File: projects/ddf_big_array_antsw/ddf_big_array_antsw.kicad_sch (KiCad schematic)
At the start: 35 parts, among them J1 Conn_Coaxial, J2 Conn_Coaxial, J3 Conn_Coaxial, J4 Conn_Coaxial, J5 Conn_Coaxial, J6 RJ45_Shielded

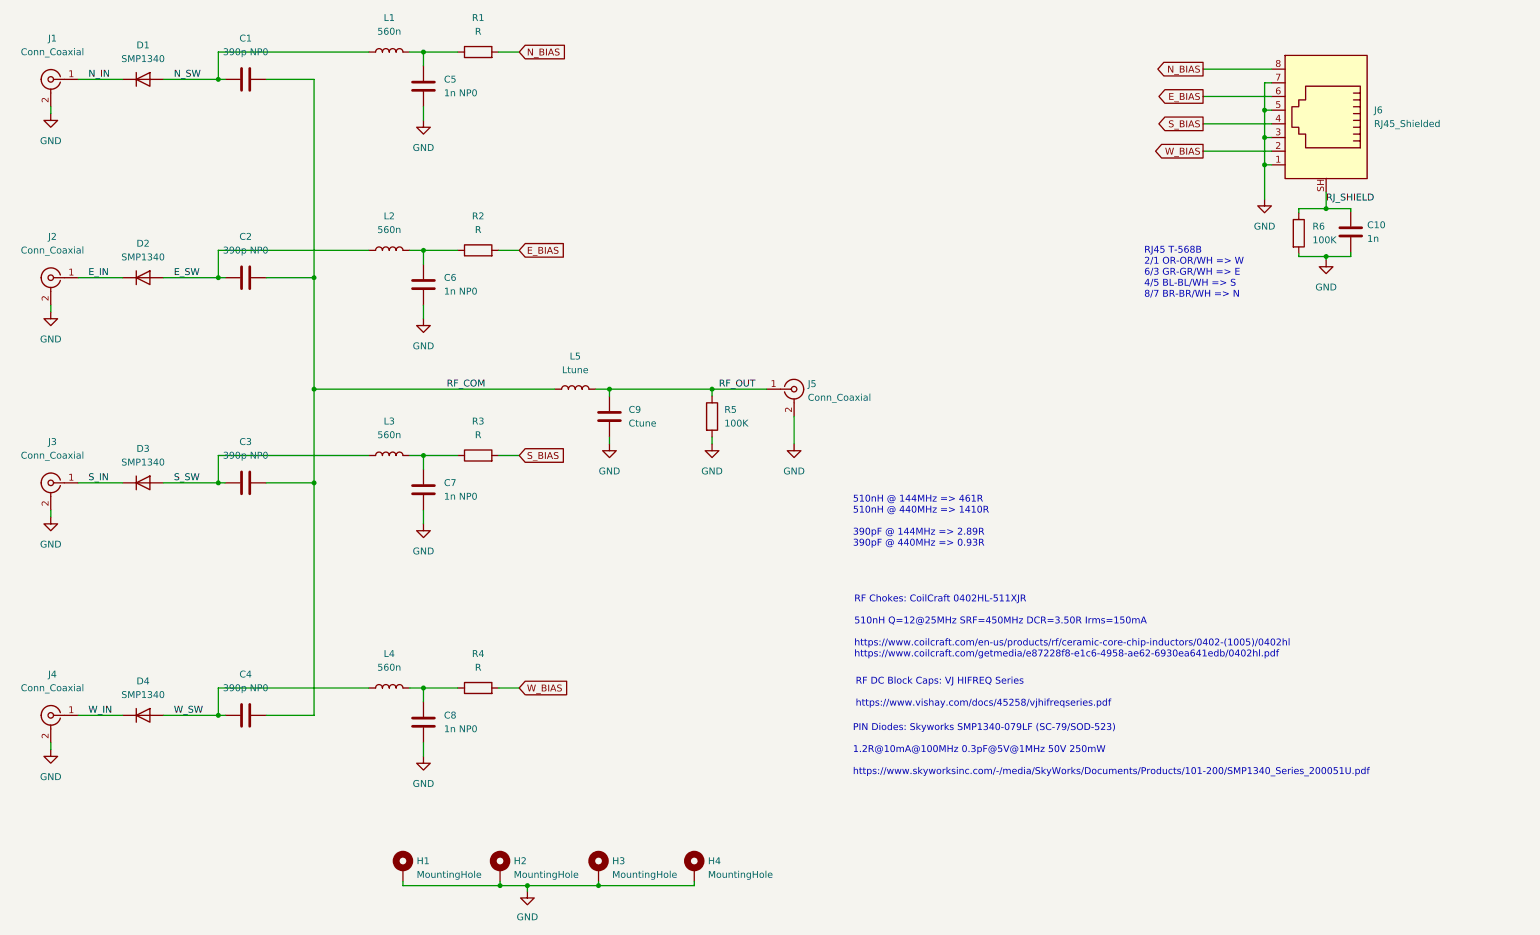
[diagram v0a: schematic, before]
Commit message: checkpoint
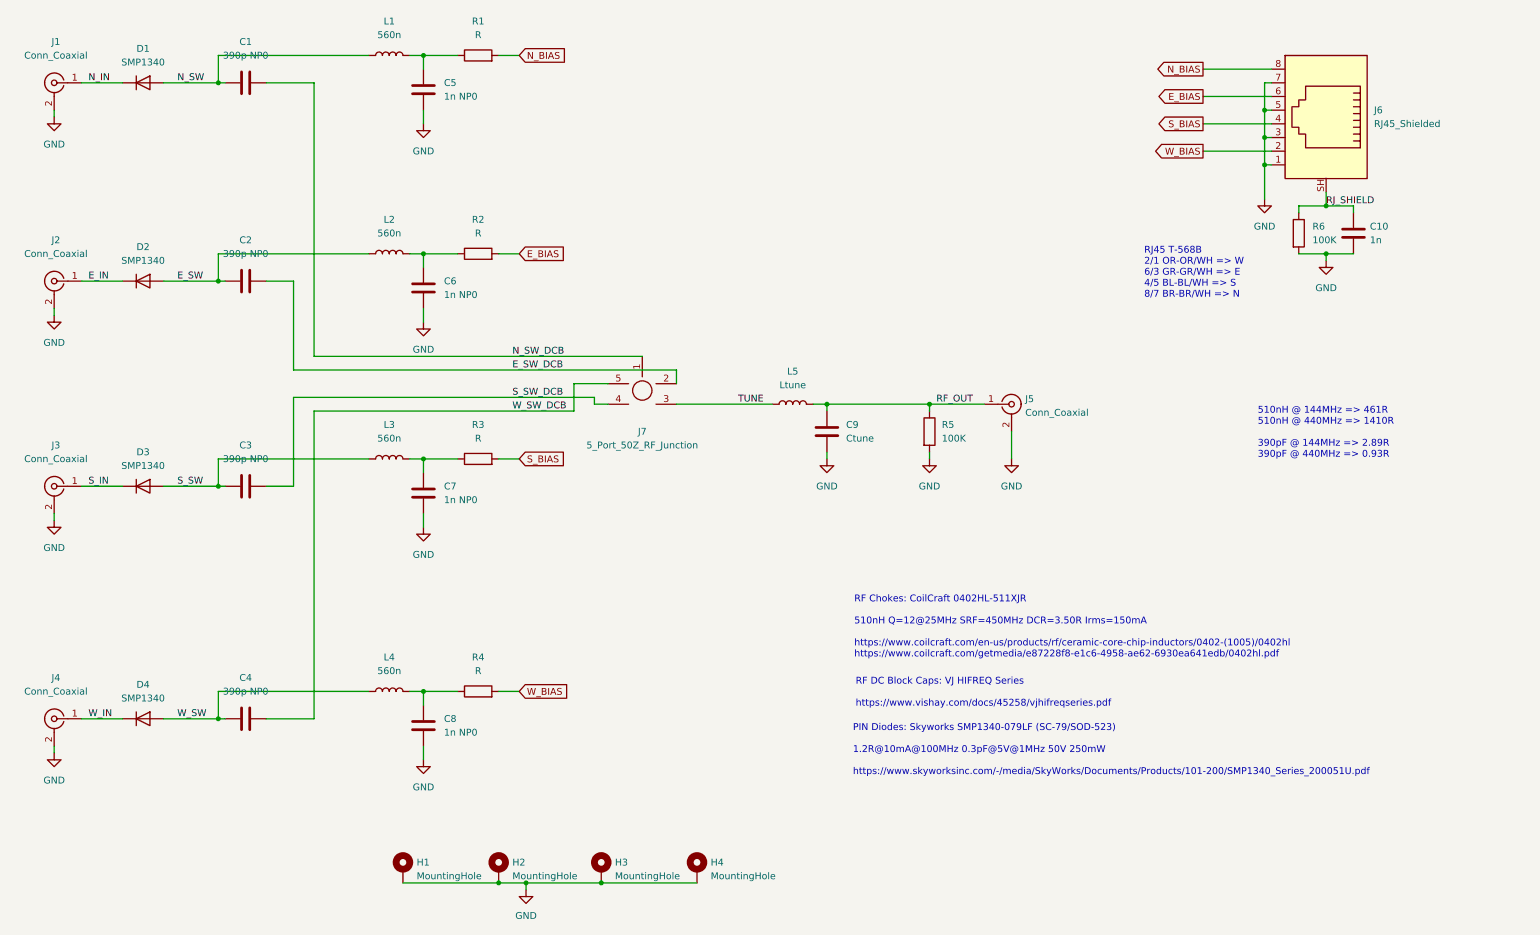
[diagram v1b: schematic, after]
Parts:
- added J7: 5_Port_50Z_RF_Junction, ch:5 Port 50Z RF Junction, symbol ch:5_Port_50Z_RF_Junction
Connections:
- removed net RF_COM: C1.2, C2.2, C3.2, C4.2, L5.1
- new net E_SW_DCB: C2.2, J7.2 (Pin_2)
- new net N_SW_DCB: C1.2, J7.1 (Pin_1)
- new net S_SW_DCB: C3.2, J7.4 (Pin_4)
- new net TUNE: J7.3 (Pin_3), L5.1
- new net W_SW_DCB: C4.2, J7.5 (Pin_5)
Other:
- moved on the sheet: C1, C10, C2, C3, C4, C5, C6, C7, C8, C9, D1, D2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
